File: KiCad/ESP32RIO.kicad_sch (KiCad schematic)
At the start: 44 parts, among them J1 Screw_Terminal_01x08, J2 Screw_Terminal_01x08, J3 Screw_Terminal_01x08, J4 Screw_Terminal_01x08, Q1 BC548, Q2 BC548, U1 PC817, U10 PC817, U11 PC817, U12 PC817, U13 PC817, U14 PC817, U15 LM7812_TO220, U16 ESP32-DEVKIT-V1, U17 XTR115U, U18 XTR115U, U19 PCF8574, U2 PC817, U20 ULN2803A, U21 TB67H451FNG, U22 SP3485CN, U3 PC817, U4 PC817, U5 PC817, U6 PC817, U7 PC817, U8 PC817, U9 PC817

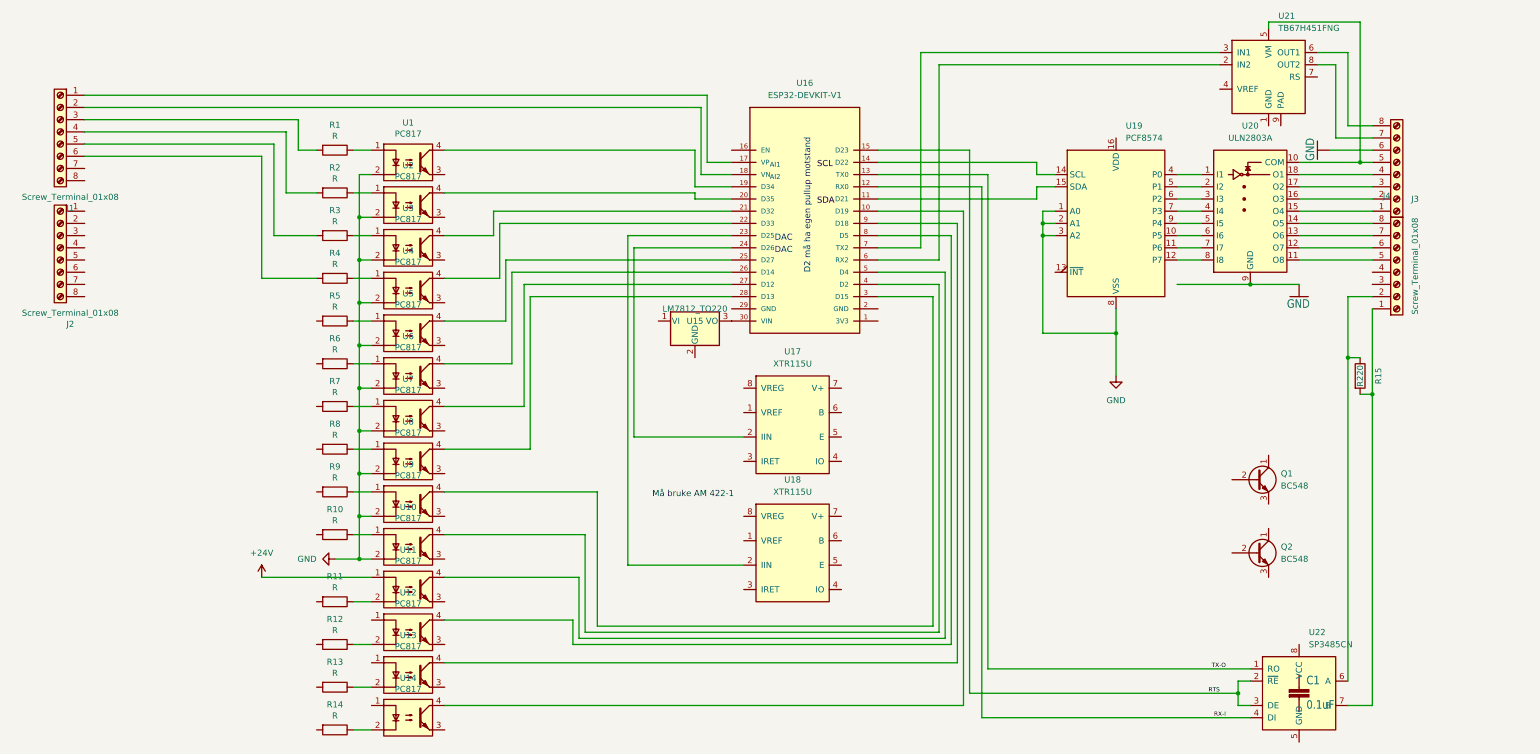
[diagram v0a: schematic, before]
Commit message: Versjon1
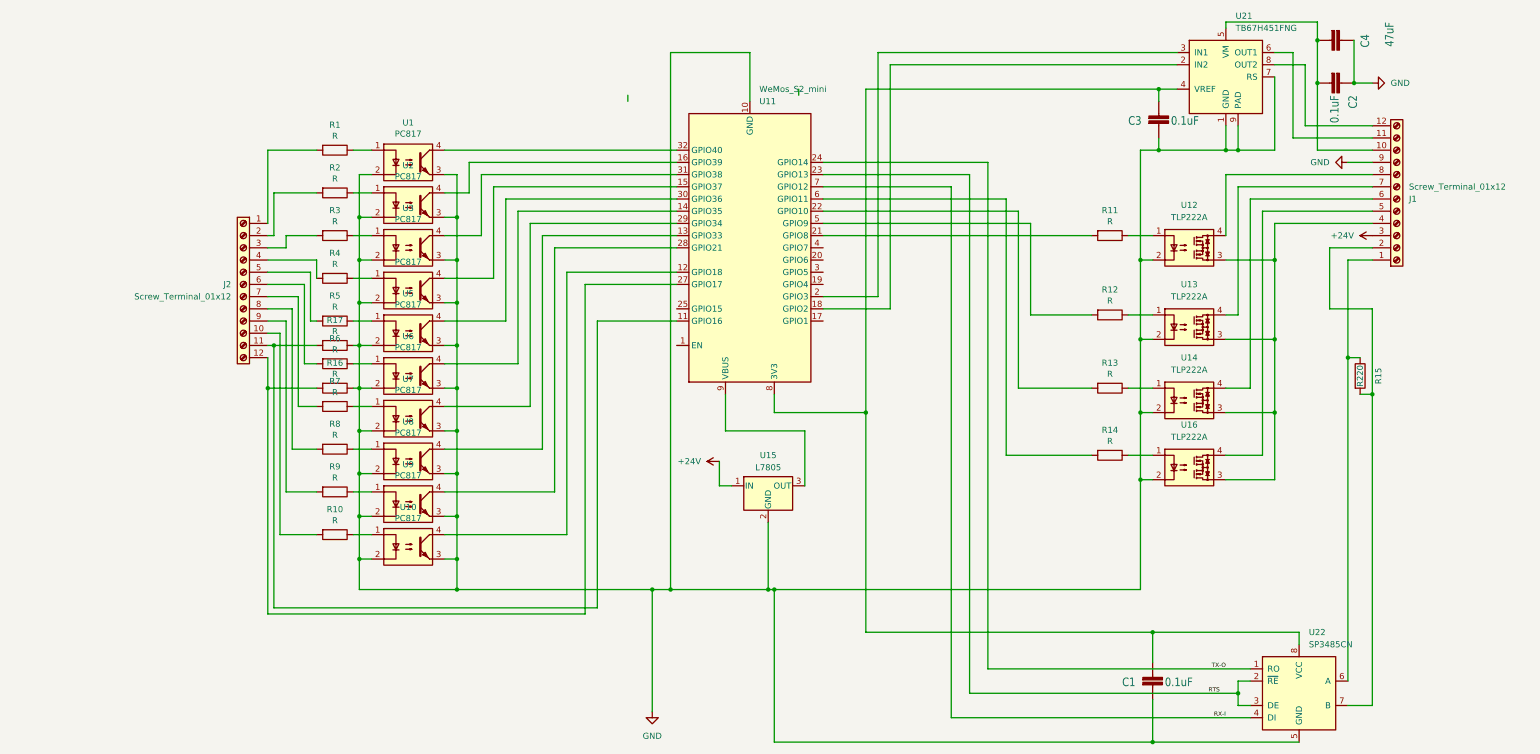
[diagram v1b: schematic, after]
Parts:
- removed J1, J2, J3, J4: Screw_Terminal_01x08, TerminalBlock_Phoenix:TerminalBlock_Phoenix_MKDS-1,5-8-5.08_1x08_P5.08mm_Horizontal, symbol Connector:Screw_Terminal_01x08
- removed Q1, Q2: BC548, Package_TO_SOT_THT:TO-92_Inline, symbol Transistor_BJT:BC548
- removed U11, U12, U13, U14: PC817, Package_DIP:DIP-4_W7.62mm, symbol Isolator:PC817
- removed U15: LM7812_TO220, Package_TO_SOT_THT:TO-220-3_Vertical, symbol Regulator_Linear:LM7812_TO220
- removed U16: ESP32-DEVKIT-V1, doit-esp32-devkit-kicad:ESP32-DOIT-DEVKIT, symbol Devkit V1-1:ESP32-DEVKIT-V1
- removed U17, U18: XTR115U, Package_SO:SOIC-8_3.9x4.9mm_P1.27mm, symbol Interface_CurrentLoop:XTR115U
- removed U19: PCF8574, Package_DIP:DIP-18_W7.62mm, symbol Interface_Expansion:PCF8574
- removed U20: ULN2803A, Package_DIP:DIP-18_W7.62mm, symbol Transistor_Array:ULN2803A
- added C2, C3: 0.1uF, Capacitor_SMD:C_1206_3216Metric_Pad1.33x1.80mm_HandSolder, symbol RS485_Breakout-eagle-import:0.1UF-25V(+80/-20%)(0603)
- added C4: 47uF, Capacitor_THT:CP_Radial_D4.0mm_P2.00mm, symbol RS485_Breakout-eagle-import:0.1UF-25V(+80/-20%)(0603)
- added J1, J2: Screw_Terminal_01x12, TerminalBlock_Phoenix:TerminalBlock_Phoenix_MKDS-1,5-12_1x12_P5.00mm_Horizontal, symbol Connector:Screw_Terminal_01x12
- added R16, R17: R, Resistor_THT:R_Axial_DIN0204_L3.6mm_D1.6mm_P2.54mm_Vertical, symbol Device:R
- added U11: WeMos_S2_mini, wemos 2s mini:WEMOS_S2_mini, symbol Wemos s2 mini:WeMos_S2_mini
- added U12, U13, U14, U16: TLP222A, Package_DIP:DIP-4_W7.62mm, symbol Relay_SolidState:TLP222A
- added U15: L7805, Package_TO_SOT_SMD:TO-263-2, symbol Regulator_Linear:L7805
- C1: footprint RS485_Breakout:0603-CAP -> Capacitor_SMD:C_1206_3216Metric_Pad1.33x1.80mm_HandSolder
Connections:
- net +24V: now also J1.3 (Pin_3), U15.1 (IN)
- net GND: now also C1.2, U1.3, U10.3, U2.3, U21.1 (GND), U21.7 (RS), U21.9 (PAD), U22.5 (GND), U3.3, U4.3, U5.3, U6.3, U7.3, U8.3, U9.3, C2.1, C3.2, C4.1, J1.9 (Pin_9), R16.1, R17.1, U11.10 (GND), U11.26 (GND), U12.2, U13.2, U14.2, U15.2 (GND), U16.2
- net RTS: now also U11.23 (GPIO13)
- net RX-I: now also U11.7 (GPIO12)
- net TX-O: now also U11.24 (GPIO14)
- net at R4.2: now also J2.4 (Pin_4)
- net at R6.2: now also J2.6 (Pin_6)
- net at R15.1, U22.6 (A): now also J1.1 (Pin_1)
- net at R15.2, U22.7 (B): now also J1.2 (Pin_2)
- net at U10.4: now also U11.12 (GPIO18)
- net at R7.2: now also J2.7 (Pin_7)
- net at U6.4: now also U11.14 (GPIO35)
- net at U3.4: now also U11.31 (GPIO38)
- net at R13.1: now also U14.1
- net at C1.1: now also U21.4 (VREF), U22.8 (VCC), C3.1, U11.8 (3V3)
- net at R2.2: now also J2.2 (Pin_2)
- net at R13.2: now also U11.22 (GPIO10)
- net at R14.1: now also U16.1
- net at R14.2: now also U11.6 (GPIO11)
- net at R9.2: now also J2.9 (Pin_9)
- net at U7.4: now also U11.29 (GPIO34)
- net at U21.5 (VM): now also C2.2, C4.2, J1.10 (Pin_10)
- net at U21.8 (OUT2): now also J1.12 (Pin_12)
- net at U21.6 (OUT1): now also J1.11 (Pin_11)
- net at R12.1: now also U13.1
- net at R8.2: now also J2.8 (Pin_8)
- net at U4.4: now also U11.15 (GPIO37)
- net at R12.2: now also U11.5 (GPIO9)
- net at U1.4: now also U11.32 (GPIO40)
- net at R10.2: now also J2.10 (Pin_10)
- net at R11.1: now also U12.1
- net at R5.2: now also J2.5 (Pin_5)
- net at U2.4: now also U11.16 (GPIO39)
- net at U21.2 (IN2): now also U11.18 (GPIO2)
- net at U21.3 (IN1): now also U11.2 (GPIO3)
- net at R1.2: now also J2.1 (Pin_1)
- net at U9.4: now also U11.28 (GPIO21)
- net at R3.2: now also J2.3 (Pin_3)
- net at U8.4: now also U11.13 (GPIO33)
- net at R11.2: now also U11.21 (GPIO8)
- net at U5.4: now also U11.30 (GPIO36)
- new net: J2.12 (Pin_12), R16.2, U11.27 (GPIO17)
- new net: J2.11 (Pin_11), R17.2, U11.11 (GPIO16)
- new net: U11.9 (VBUS), U15.3 (OUT)
- new net: J1.4 (Pin_4), U12.3, U13.3, U14.3, U16.3
- new net: J1.5 (Pin_5), U16.4
- new net: J1.6 (Pin_6), U14.4
- new net: J1.7 (Pin_7), U13.4
- new net: J1.8 (Pin_8), U12.4
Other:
- note removed: "AI1"
- note removed: "AI2"
- note removed: "D2 må ha egen pullup motstand"
- note removed: "DAC"
- note removed: "Må bruke AM 422-1"
- moved on the sheet: C1, U21
